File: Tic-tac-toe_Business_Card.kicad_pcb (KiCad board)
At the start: 2 copper layers, 85 x 55 mm, 81 parts, among them J1 USB_C_Receptacle_USB2.0_14P, J2 Conn_01x04, SW1 SW_Push, SW2 SW_Push, SW3 SW_Push, U1 MCP1700x-330xxTT, U3 W25Q16JVUXIQ TR, U4 RP2040, U5 NT3H2111W0FHKH, Y1 12 MHz

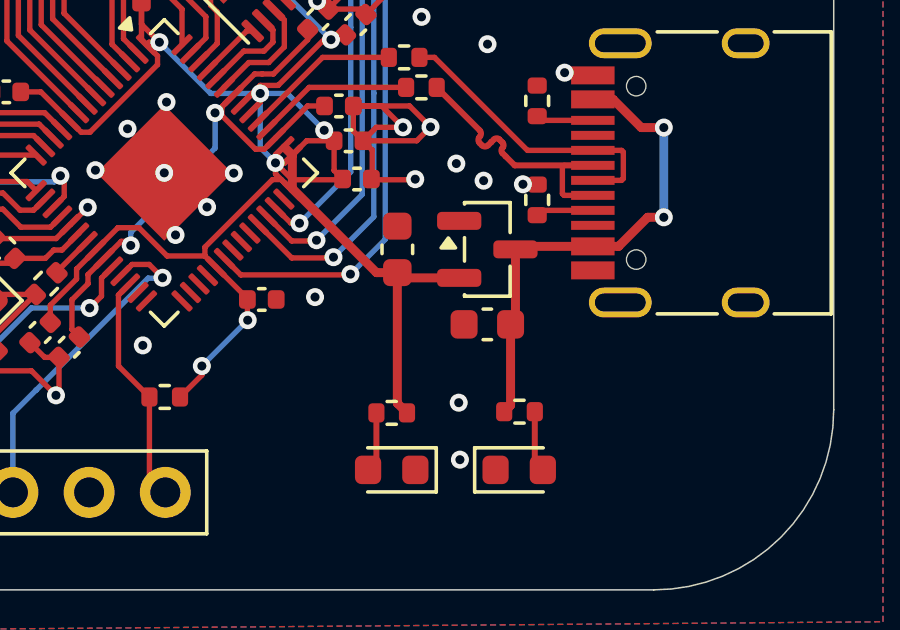
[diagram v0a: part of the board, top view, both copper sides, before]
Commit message: Update Repo
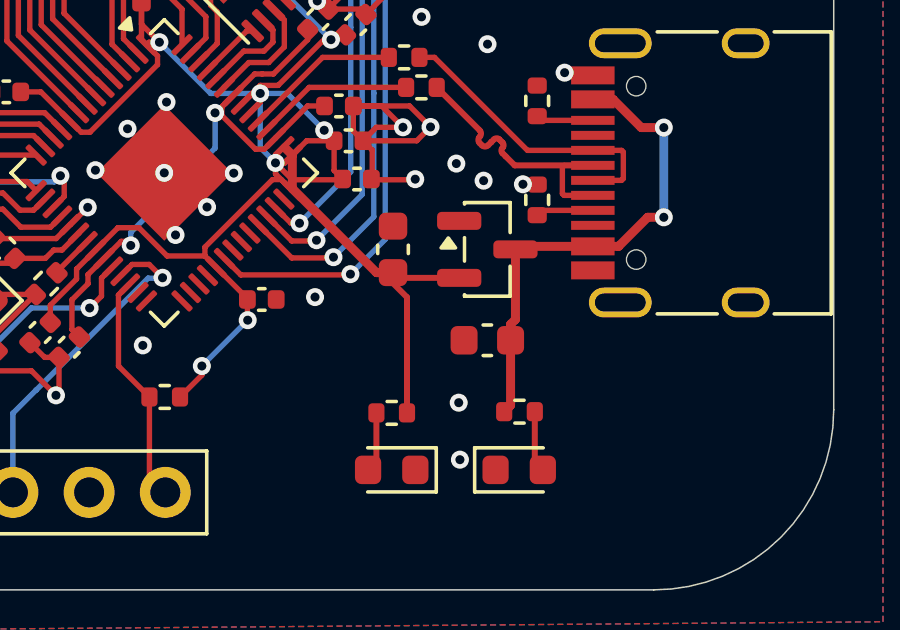
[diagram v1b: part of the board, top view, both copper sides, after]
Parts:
- C13, C17: value 33pF -> 15pF
- moved C2 0.53 mm to (95.8, 67.3)
- moved C3 0.14 mm to (92.7, 64.3)
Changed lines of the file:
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@@
 	(footprint "Capacitor_SMD:C_0603_1608Metric"
 		(layer "F.Cu")
-		(at 95.843359 66.77 180)
+		(at 95.843359 67.3 180)
 		(descr "Capacitor SMD 0603 (1608 Metric), square (rectangular) end terminal, IPC-7351 nominal, (Body size source: IPC-SM-782 page 76, https://www.pcb-3d.com/wordpress/wp-content/uploads/ipc-sm-782a_amendment_1_and_2.pdf), generated with kicad-footprint-generator")
 		(tags "capacitor")
@@
 	(footprint "Capacitor_SMD:C_0603_1608Metric"
 		(layer "F.Cu")
-		(at 92.843359 64.27 90)
+		(at 92.7 64.27 90)
 		(descr "Capacitor SMD 0603 (1608 Metric), square (rectangular) end terminal, IPC-7351 nominal, (Body size source: IPC-SM-782 page 76, https://www.pcb-3d.com/wordpress/wp-content/uploads/ipc-sm-782a_amendment_1_and_2.pdf), generated with kicad-footprint-generator")
 		(tags "capacitor")
@@
 			)
 		)
-		(property "Value" "33pF"
+		(property "Value" "15pF"
 			(at 0 1.16 45)
 			(layer "F.Fab")
@@
 			)
 		)
-		(property "Value" "33pF"
+		(property "Value" "15pF"
 			(at 0 1.16 135)
 			(layer "F.Fab")
@@
 	)
 	(segment
+		(start 92.6 65.045)
+		(end 92.6 65.3)
+		(width 0.2)
+		(layer "F.Cu")
+		(net 3)
+	)
+	(segment
 		(start 80.960275 59.02)
 		(end 81.936702 59.996427)
@@
 	)
 	(segment
+		(start 92.775 65.22)
+		(end 92.6 65.045)
+		(width 0.2)
+		(layer "F.Cu")
+		(net 3)
+	)
+	(segment
 		(start 89.870489 55.140624)
 		(end 89.083816 55.927297)
@@
 	)
 	(segment
-		(start 94.905859 65.22)
-		(end 93.018359 65.22)
-		(width 0.3)
-		(layer "F.Cu")
-		(net 3)
-	)
-	(segment
 		(start 91.045859 61.95)
 		(end 89.344403 61.95)
@@
 	)
 	(segment
-		(start 92.843359 69.3975)
-		(end 93.165859 69.72)
-		(width 0.3)
-		(layer "F.Cu")
-		(net 3)
-	)
-	(segment
 		(start 84.912878 57.365252)
 		(end 84.567877 57.365252)
@@
 	)
 	(segment
+		(start 92.6 65.3)
+		(end 93.165859 65.865859)
+		(width 0.2)
+		(layer "F.Cu")
+		(net 3)
+	)
+	(segment
 		(start 82.151403 64.925928)
 		(end 82.151403 65.258542)
@@
 	)
 	(segment
-		(start 93.018359 65.22)
-		(end 92.843359 65.045)
-		(width 0.3)
-		(layer "F.Cu")
-		(net 3)
-	)
-	(segment
 		(start 82.78523 64.292101)
 		(end 82.151403 64.925928)
@@
 	)
 	(segment
+		(start 93.165859 65.865859)
+		(end 93.165859 69.72)
+		(width 0.2)
+		(layer "F.Cu")
+		(net 3)
+	)
+	(segment
 		(start 84.850782 57.819339)
 		(end 84.850782 58.112603)
@@
 	)
 	(segment
+		(start 93.1 69.654141)
+		(end 93.165859 69.72)
+		(width 0.2)
+		(layer "F.Cu")
+		(net 3)
+	)
+	(segment
 		(start 90.556082 57.119411)
 		(end 90.556082 57.2044)
@@
 	)
 	(segment
-		(start 92.843359 65.045)
-		(end 92.843359 69.3975)
-		(width 0.3)
-		(layer "F.Cu")
-		(net 3)
-	)
-	(segment
 		(start 90.556082 57.119411)
 		(end 91.116448 57.119411)
@@
 		(layer "F.Cu")
 		(net 3)
+	)
+	(segment
+		(start 94.905859 65.22)
+		(end 92.775 65.22)
+		(width 0.2)
+		(layer "F.Cu")
+		(net 3)
